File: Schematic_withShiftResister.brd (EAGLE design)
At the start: 83.8 x 80.2 mm, 31 parts, among them U1 328P, U2 SN74HC595D, U3 3.3V/150mA, U4 SN74HC595D

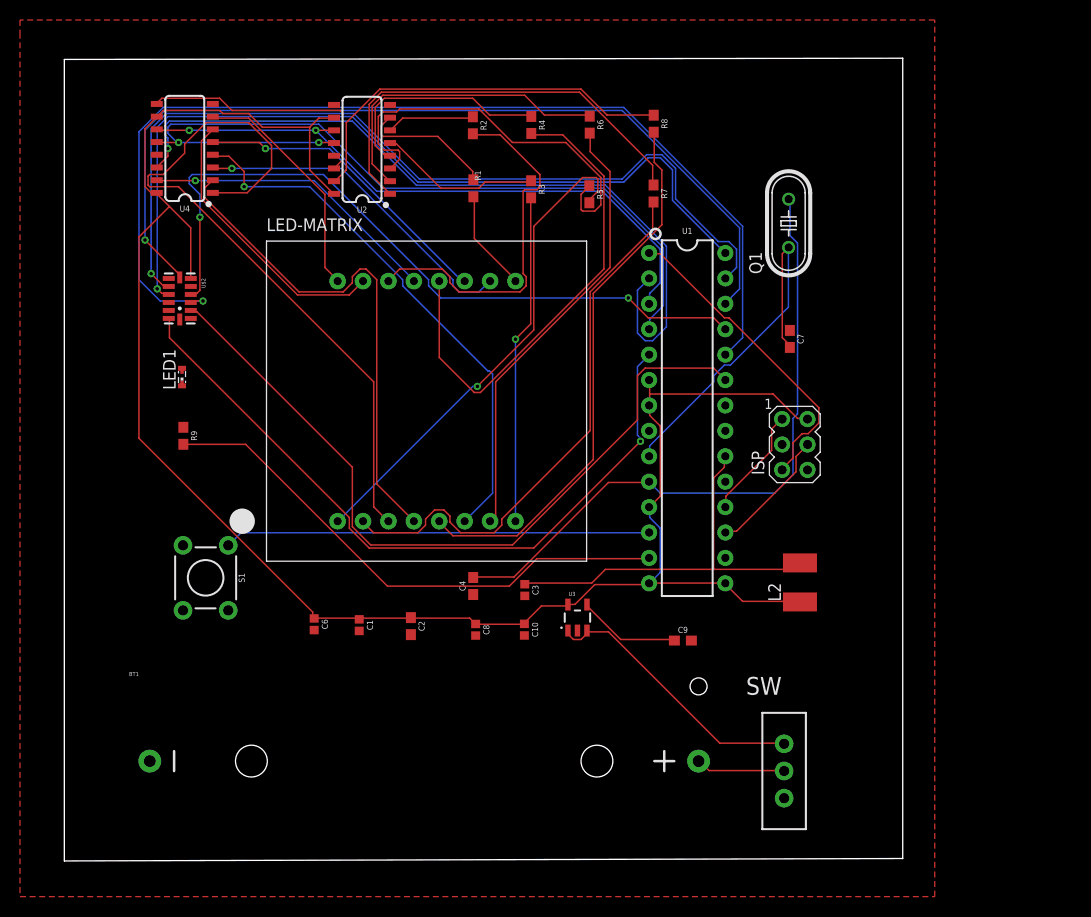
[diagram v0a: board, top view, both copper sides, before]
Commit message: Add files via upload
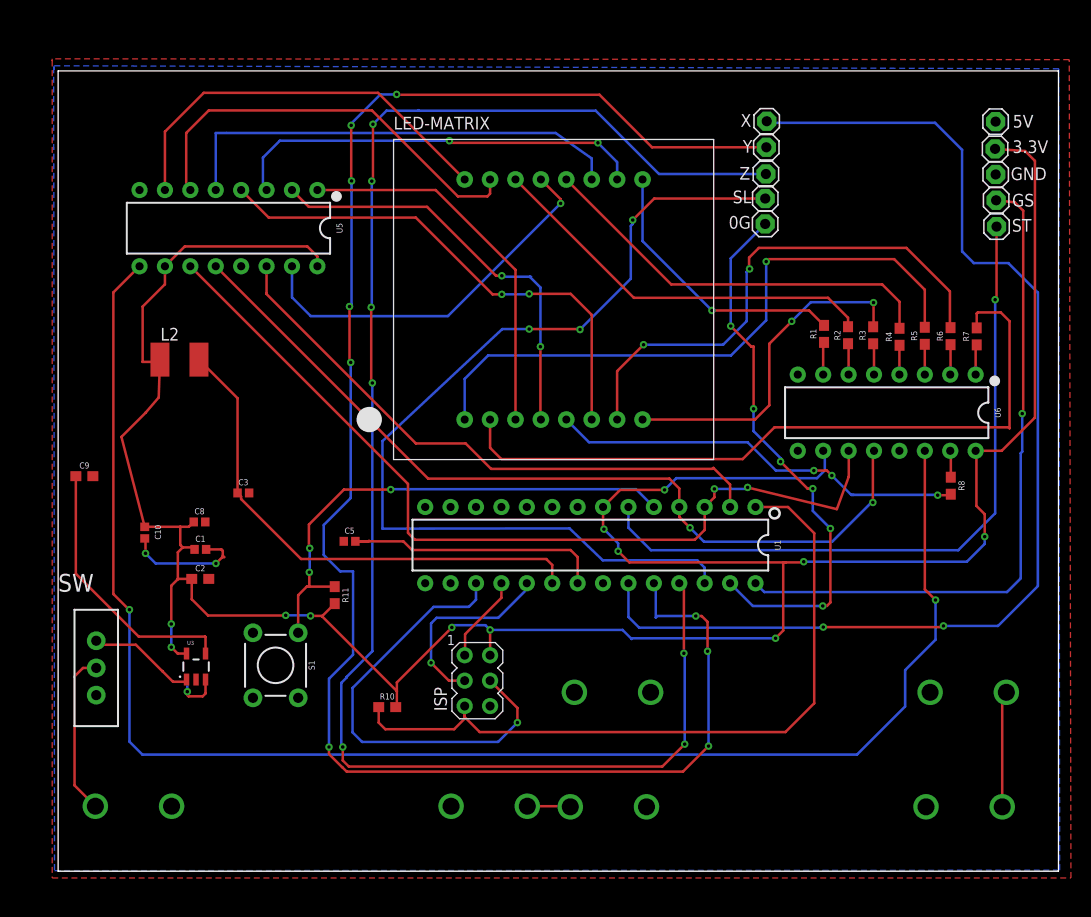
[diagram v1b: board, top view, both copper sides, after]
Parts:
- removed C4, C7: 22pF, SparkFun-Capacitors:0603
- removed C6: 0.1uF, SparkFun-Capacitors:0402
- removed LED1: (no value), adafruit:SMARTLED-TTW
- removed Q1: (no value), adafruit:HC49/S
- removed R9: 150, SparkFun-Resistors:0603
- removed U$2: MMA7361, SparkFun:LGA14
- removed U2, U4: SN74HC595D, SparkFun-IC-Logic:SO16
- added 0G, 3.3V, 5V, GND, GS, SL, ST, X, Y, Z: (no value), adafruit:1X01
- added BT2, BT3: (no value), SparkFun-Batteries:BATTERY-AAA-KIT
- added C5: 0.1uF, SparkFun-Capacitors:0402
- added R10, R11: 10k, SparkFun-Resistors:0603
- added U5, U6: SN74HC595N, SparkFun-IC-Logic:DIP16
- BT1: device SparkFun-Retired:BATTERY-AA-PANEL -> SparkFun-Batteries:BATTERY-AAA-KIT
- moved SW 69.5 mm to (3.81, 20.3)
- moved L2 65.9 mm to (12.1, 51.1), turned to 0 degrees
- moved C9 62.0 mm to (2.62, 39.5)
- moved R8 46.8 mm to (89.2, 38.5)
- moved R2 43.0 mm to (79.0, 53.6), turned to 90 degrees
- moved R4 42.5 mm to (84.1, 53.4), turned to 90 degrees
- moved R6 41.8 mm to (89.2, 53.5), turned to 90 degrees
- moved ISP 39.5 mm to (41.9, 19.1)
- moved C10 39.2 mm to (8.66, 33.8)
- moved U3 38.4 mm to (13.8, 20.5)
- moved R1 38.0 mm to (76.6, 53.7), turned to 90 degrees
- moved R3 37.2 mm to (81.5, 53.6), turned to 90 degrees
- moved R5 36.4 mm to (86.6, 53.5), turned to 90 degrees
- moved R7 35.3 mm to (91.8, 53.5), turned to 90 degrees
- moved C3 29.8 mm to (18.5, 37.8), turned to 0 degrees
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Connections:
- removed net +3.3V: C1.1, C10.1, C2.1, C6.1, C8.1, ISP.2, L2.1, U$2.6, U1.11, U1.14, U1.15, U1.6, U1.7, U2.10, U2.16, U3.5, U4.10, U4.16
- removed net N$37: R9.2, U1.13
- removed net N$39: LED1.A@1, R9.1
- removed net N$44: U$2.10, U1.28
- new net 3.3V: 3.3V.1, C1.1, C10.1, C2.1, C8.1, ISP.2, L2.1, R10.2, R11.2, U1.7, U3.5, U5.10, U5.16, U6.10, U6.16
- new net N$46: ST.1, U1.6
- net GND: now also 5V.1, BT3.GND@1, C5.1, GND.1, U5.13, U5.8, U6.13, U6.8; no longer BT1.-, C4.1, C6.2, C7.1, LED1.C@1, U$2.5, U2.13, U2.8, U4.13, U4.8
- net N$10: now also U5.2; no longer U4.2
- net N$11: now also U5.3; no longer U4.3
- net N$12: now also U5.4; no longer U4.4
- net N$13: now also U5.5; no longer U4.5
- net N$14: now also U5.6; no longer U4.6
- net N$15: now also U5.7; no longer U4.7
- net N$16: now also U6.15; no longer U2.15
- net N$17: now also X.1; no longer U$2.2
- net N$18: now also Y.1; no longer U$2.3
- net N$19: now also Z.1; no longer U$2.4
- net N$20: now also U6.1; no longer U2.1
- net N$21: now also U6.2; no longer U2.2
- net N$22: now also U6.3; no longer U2.3
- net N$23: now also U6.4; no longer U2.4
- net N$24: now also U6.5; no longer U2.5
- net N$25: now also U6.6; no longer U2.6
- net N$26: now also U6.7; no longer U2.7
- net N$27: now also U5.1; no longer U4.1
- net N$28: now also U5.11, U6.11; no longer U2.11, U4.11
- net N$30: now also BT2.GND@1, BT3.PWR@1; no longer C4.2, Q1.2, U1.10
- net N$31: now also BT1.GND@1, BT2.PWR@1; no longer C7.2, Q1.1, U1.9
- net N$33: now also U5.14; no longer U4.14
- net N$34: now also U5.9, U6.14; no longer U2.14, U4.9
- net N$35: now also U5.12, U6.12; no longer U2.12, U4.12
- net N$36: now also BT1.PWR@1; no longer BT1.+
- net N$38: now also C5.2, U1.21; no longer U1.19
- net N$40: now also R11.1, U1.5; no longer U1.12
- net N$41: now also SL.1; no longer U$2.7
- net N$42: now also 0G.1; no longer U$2.9
- net N$45: now also GS.1, U1.28; no longer U$2.13, U1.5
- net N$9: now also U5.15; no longer U4.15
- net RESET: now also R10.1
- net SCK: now also U1.19
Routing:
- net 3.3V: track 0.00 -> 268.2 mm, vias 0 -> 12
- net +3.3V: track 186.0 -> 0.00 mm
- net N$34: track 25.4 -> 156.6 mm, vias 0 -> 2
- net N$19: track 73.3 -> 159.3 mm, vias 2 -> 7
- net N$44: track 84.2 -> 0.00 mm, vias 1 -> 0
- net N$18: track 103.2 -> 173.3 mm, vias 1 -> 9
- net N$46: track 0.00 -> 69.9 mm, vias 0 -> 1
- net N$30: track 65.3 -> 11.6 mm
- net N$37: track 53.6 -> 0.00 mm
- net RESET: track 31.5 -> 73.9 mm
- net N$20: track 43.7 -> 3.01 mm
- net N$17: track 77.0 -> 115.9 mm, vias 0 -> 2
- net N$22: track 40.5 -> 3.03 mm
- net N$16: track 39.7 -> 2.66 mm
- net N$42: track 88.7 -> 55.0 mm, vias 1 -> 6
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- added copper zone on layer 16, net GND
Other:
- board size 83.8 x 80.2 mm -> 100 x 80 mm
